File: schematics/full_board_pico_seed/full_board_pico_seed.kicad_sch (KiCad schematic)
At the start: 32 parts, among them J7 Conn_02x20_Odd_Even, J8 Conn_01x03, J9 Conn_01x02_Male, P1 25k, P2 25k, P3 25k, SW4 Exit, SW5 Enter, U10 128X64 OLED Display, U6 LM1117DT-5.0, U8 AP63205WU

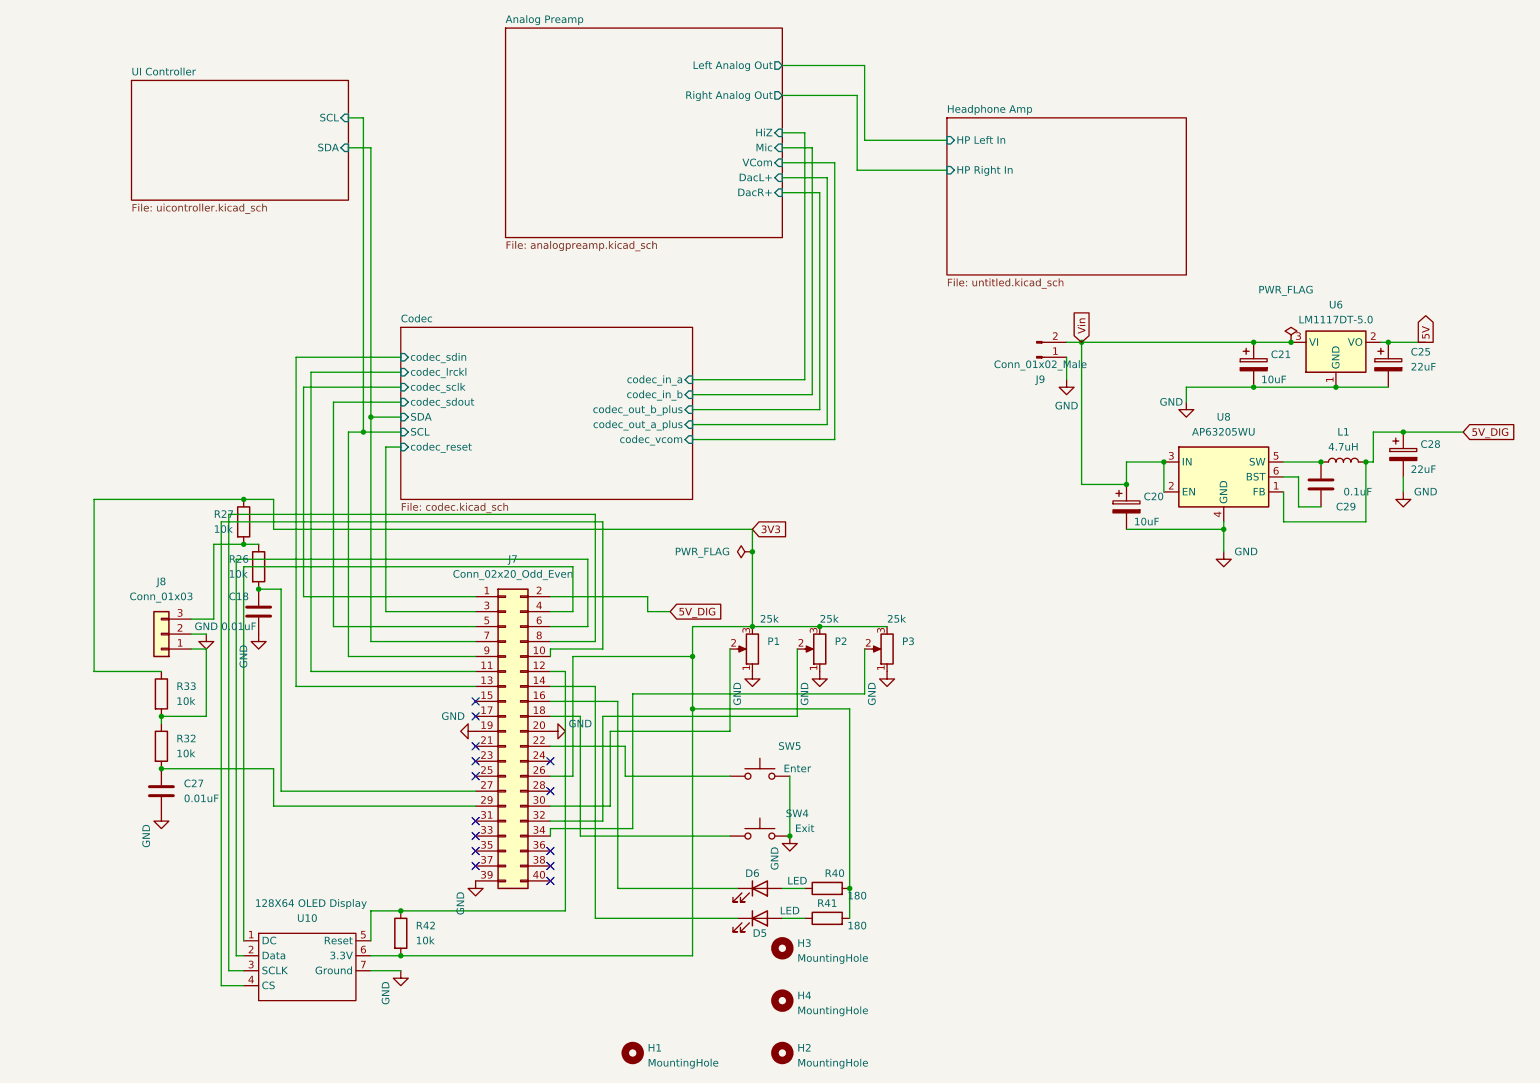
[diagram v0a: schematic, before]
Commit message: updated schematic
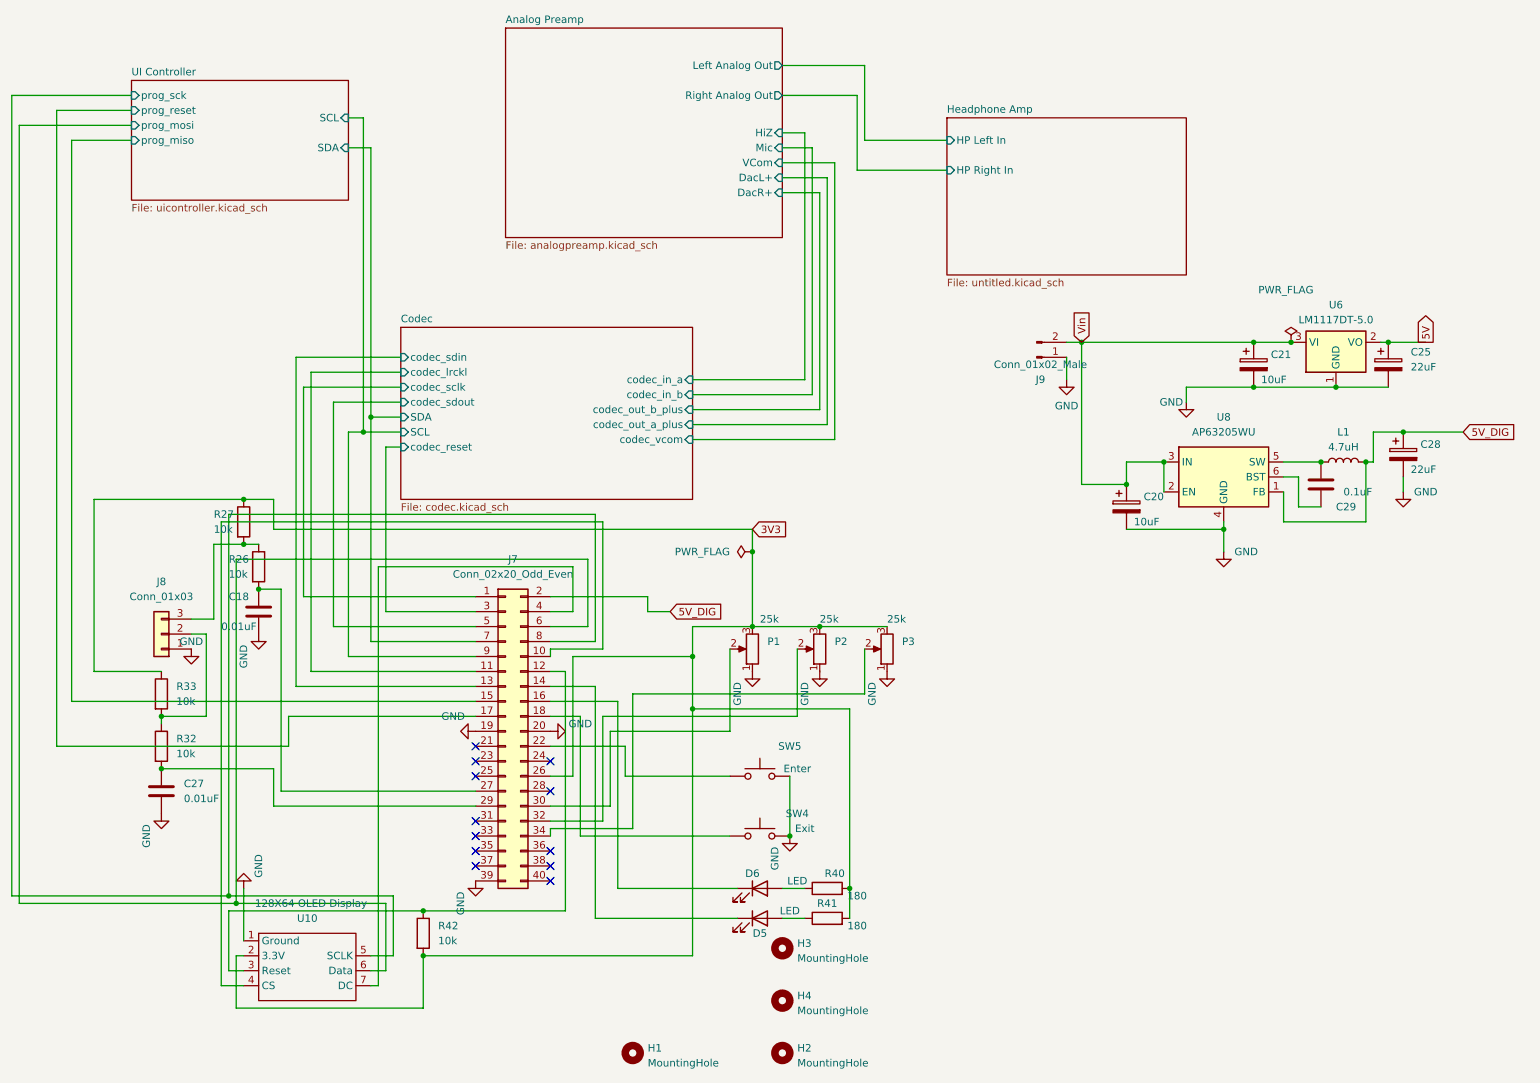
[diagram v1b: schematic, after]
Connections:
- net 3V3: now also U10.2 (3.3V); no longer U10.6 (3.3V)
- net GND: now also J8.1 (Pin_1), U10.1 (Ground); no longer J8.2 (Pin_2), U10.7 (Ground)
- net at R32.1, R33.2: now also J8.2 (Pin_2); no longer J8.1 (Pin_1)
- net at J7.12 (Pin_12), R42.1: now also U10.3 (Reset); no longer U10.5 (Reset)
- net UI Controller/prog_miso: now reaches J7.15 (Pin_15)
- net UI Controller/prog_reset: now reaches J7.17 (Pin_17)
- net at J7.4 (Pin_4): now also U10.7 (DC); no longer U10.1 (DC)
- net UI Controller/prog_mosi: now reaches J7.6 (Pin_6)
- net UI Controller/prog_mosi: now also U10.6 (Data); no longer U10.2 (Data)
- net UI Controller/prog_sck: now reaches J7.8 (Pin_8)
- net UI Controller/prog_sck: now also U10.5 (SCLK); no longer U10.3 (SCLK)
- no-connect marks 14 -> 12
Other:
- sheet UI Controller ports: added prog_miso, prog_mosi, prog_reset, prog_sck; removed none
- moved on the sheet: R42
